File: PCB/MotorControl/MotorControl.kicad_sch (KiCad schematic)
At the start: 23 parts, among them J1 Conn_01x03_Pin, J2 Conn_01x03_Pin, J3 Conn_01x03_Pin, J4 Conn_01x03_Pin, J5 Conn_01x05_Pin, J6 USB_C_Receptacle_USB2.0_14P, J7 Conn_01x03_Pin, J8 Conn_01x02_Pin, U1 PCA9685PW, U2 NORA-W106-00B, U3 TC1262-33, U4 STM32L031K6Tx

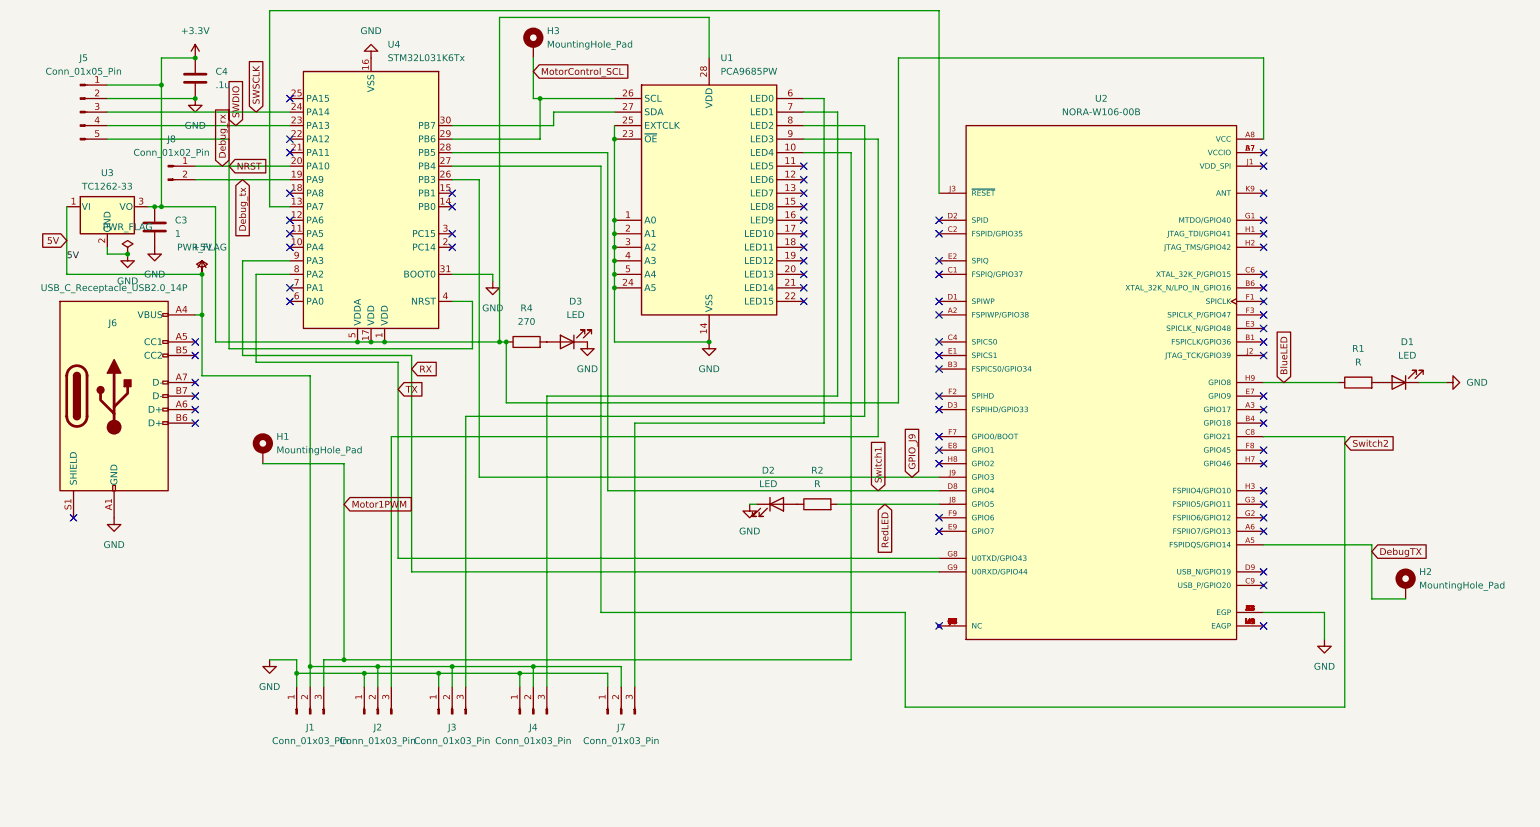
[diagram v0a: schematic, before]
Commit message: Motor
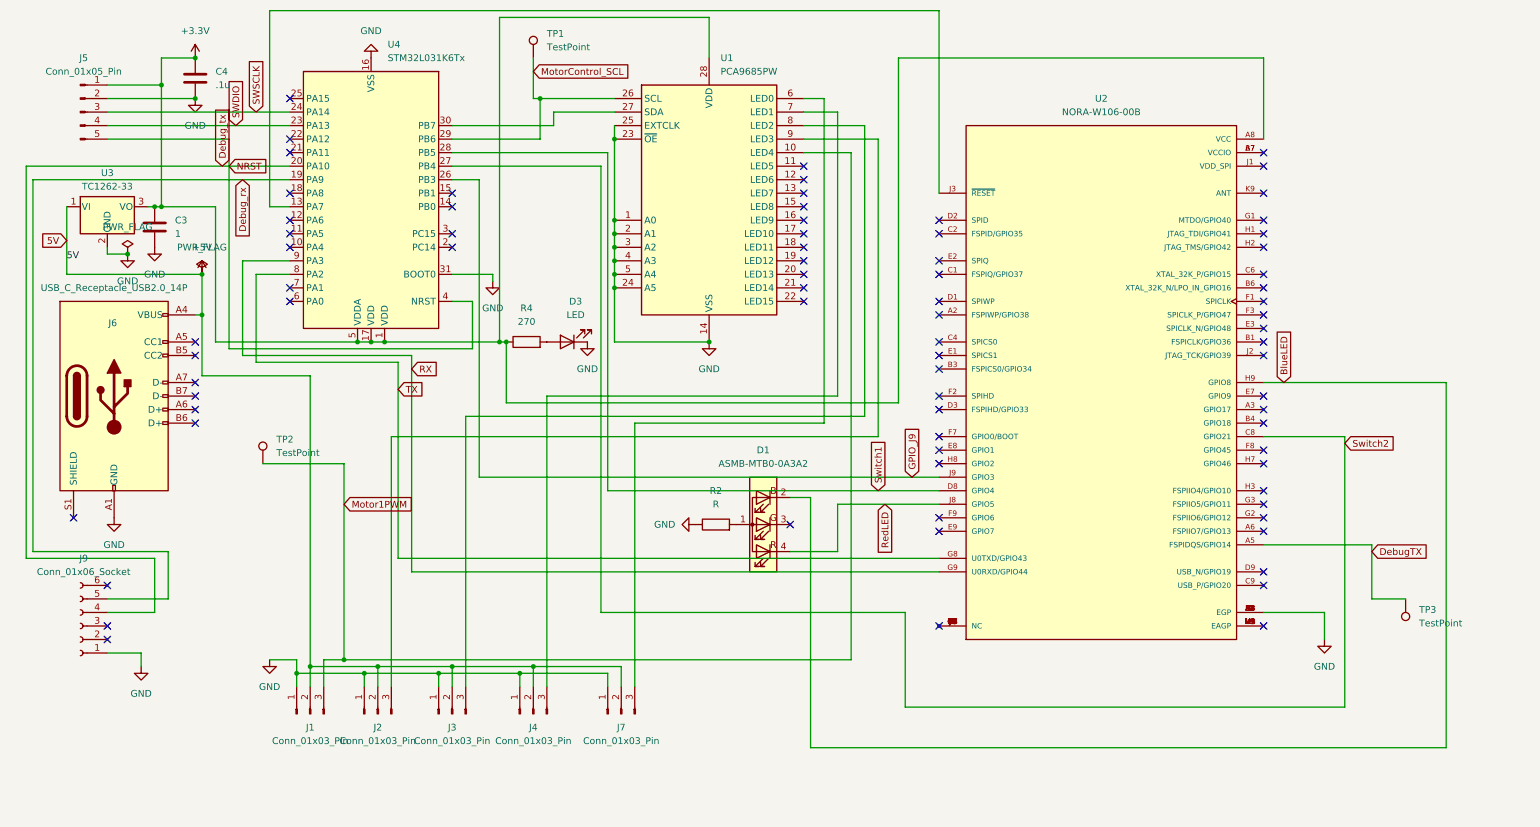
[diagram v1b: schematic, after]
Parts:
- removed D1, D2: LED, LED_SMD:LED_1206_3216Metric_Pad1.42x1.75mm_HandSolder, symbol Device:LED
- removed H1, H2, H3: MountingHole_Pad, MountingHole:MountingHole_4.5mm_Pad, symbol Mechanical:MountingHole_Pad
- removed J8: Conn_01x02_Pin, Connector_PinHeader_2.54mm:PinHeader_1x02_P2.54mm_Vertical, symbol Connector:Conn_01x02_Pin
- removed R1: R, Resistor_SMD:R_0805_2012Metric_Pad1.20x1.40mm_HandSolder, symbol Device:R
- added D1: ASMB-MTB0-0A3A2, LED_SMD:LED_Avago_PLCC4_3.2x2.8mm_CW, symbol LED:ASMB-MTB0-0A3A2
- added J9: Conn_01x06_Socket, Connector_PinSocket_2.54mm:PinSocket_1x06_P2.54mm_Vertical, symbol Connector:Conn_01x06_Socket
- added TP1, TP2, TP3: TestPoint, TestPoint:TestPoint_Pad_2.5x2.5mm, symbol Connector:TestPoint
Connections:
- net BlueLED: now also D1.2 (BK)
- net DebugTX: now also TP3.1
- net Debug_rx: now also U4.19 (PA9), J9.5 (Pin_5); no longer J5.5 (Pin_5), U4.20 (PA10), U4.4 (NRST)
- net Debug_tx: now also J5.5 (Pin_5), U4.20 (PA10), U4.4 (NRST), J9.4 (Pin_4); no longer U4.19 (PA9)
- net GND: now also R2.1, J9.1 (Pin_1)
- net Motor1PWM: now also TP2.1
- net MotorControl_SCL: now also TP1.1
- net RedLED: now also D1.4 (RK); no longer R2.2
- new net: D1.1 (A), R2.2
- no-connect marks 73 -> 77
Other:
- moved on the sheet: R2

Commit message: wasd
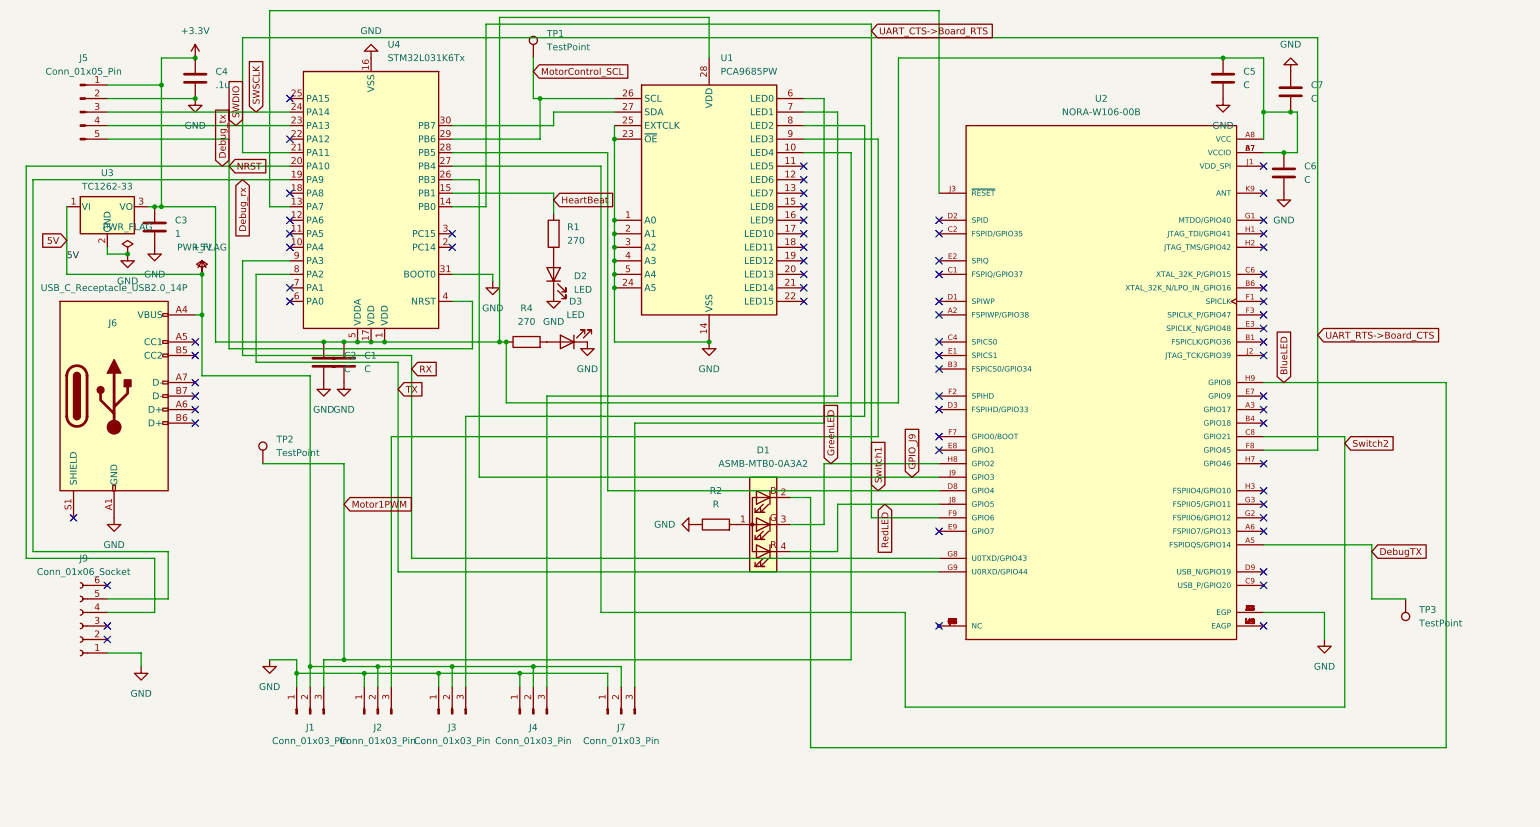
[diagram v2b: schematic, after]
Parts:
- added C1, C2, C5, C6, C7: C, Capacitor_SMD:C_0504_1310Metric_Pad0.83x1.28mm_HandSolder, symbol Device:C
- added D2: LED, LED_SMD:LED_1206_3216Metric_Pad1.42x1.75mm_HandSolder, symbol Device:LED
- added R1: 270, Resistor_SMD:R_0805_2012Metric_Pad1.20x1.40mm_HandSolder, symbol Device:R
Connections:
- net +3.3V: now also U2.A7 (VCCIO), U2.B7 (VCCIO), C1.1, C2.1, C5.1, C6.1, C7.2
- net GND: now also C1.2, C2.2, C5.2, C6.2, C7.1, D2.1 (K)
- net RX: now also U2.G8 (U0TXD/GPIO43); no longer U2.G9 (U0RXD/GPIO44)
- net TX: now also U2.G9 (U0RXD/GPIO44); no longer U2.G8 (U0TXD/GPIO43)
- net GreenLED: now reaches D1.3 (GK)
- net GreenLED: now also U2.H8 (GPIO2)
- net UART_RTS->Board_CTS: now reaches U2.F8 (GPIO45)
- net UART_RTS->Board_CTS: now also U4.21 (PA11)
- net UART_CTS->Board_RTS: now reaches U2.F9 (GPIO6)
- net UART_CTS->Board_RTS: now also U4.14 (PB0)
- net HeartBeat: now reaches U4.15 (PB1)
- net HeartBeat: now also R1.2
- new net: D2.2 (A), R1.1
- no-connect marks 77 -> 69

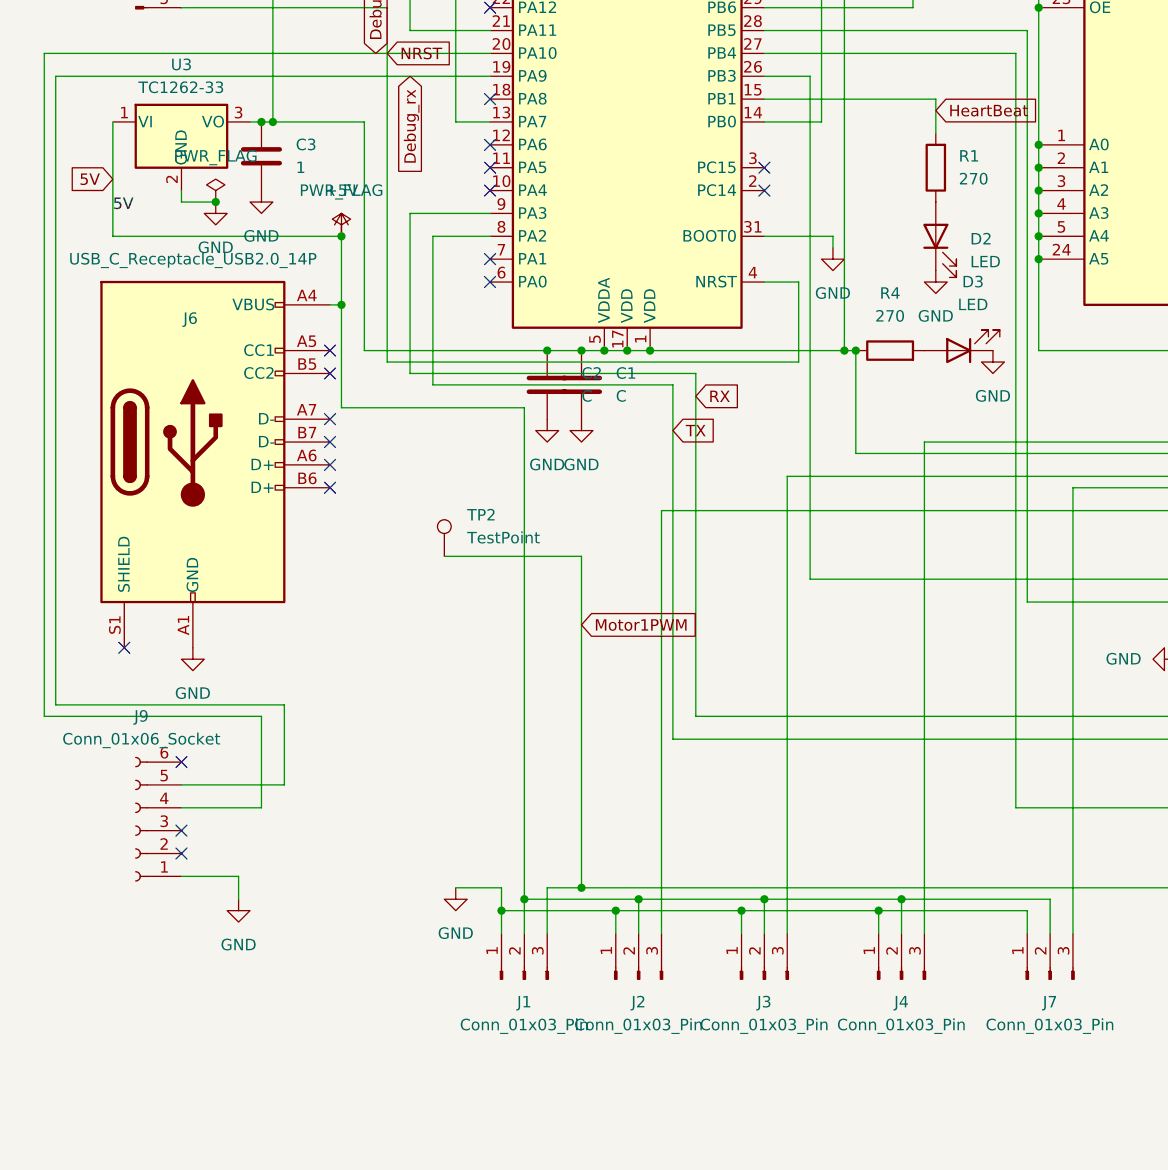
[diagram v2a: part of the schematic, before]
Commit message: wasd
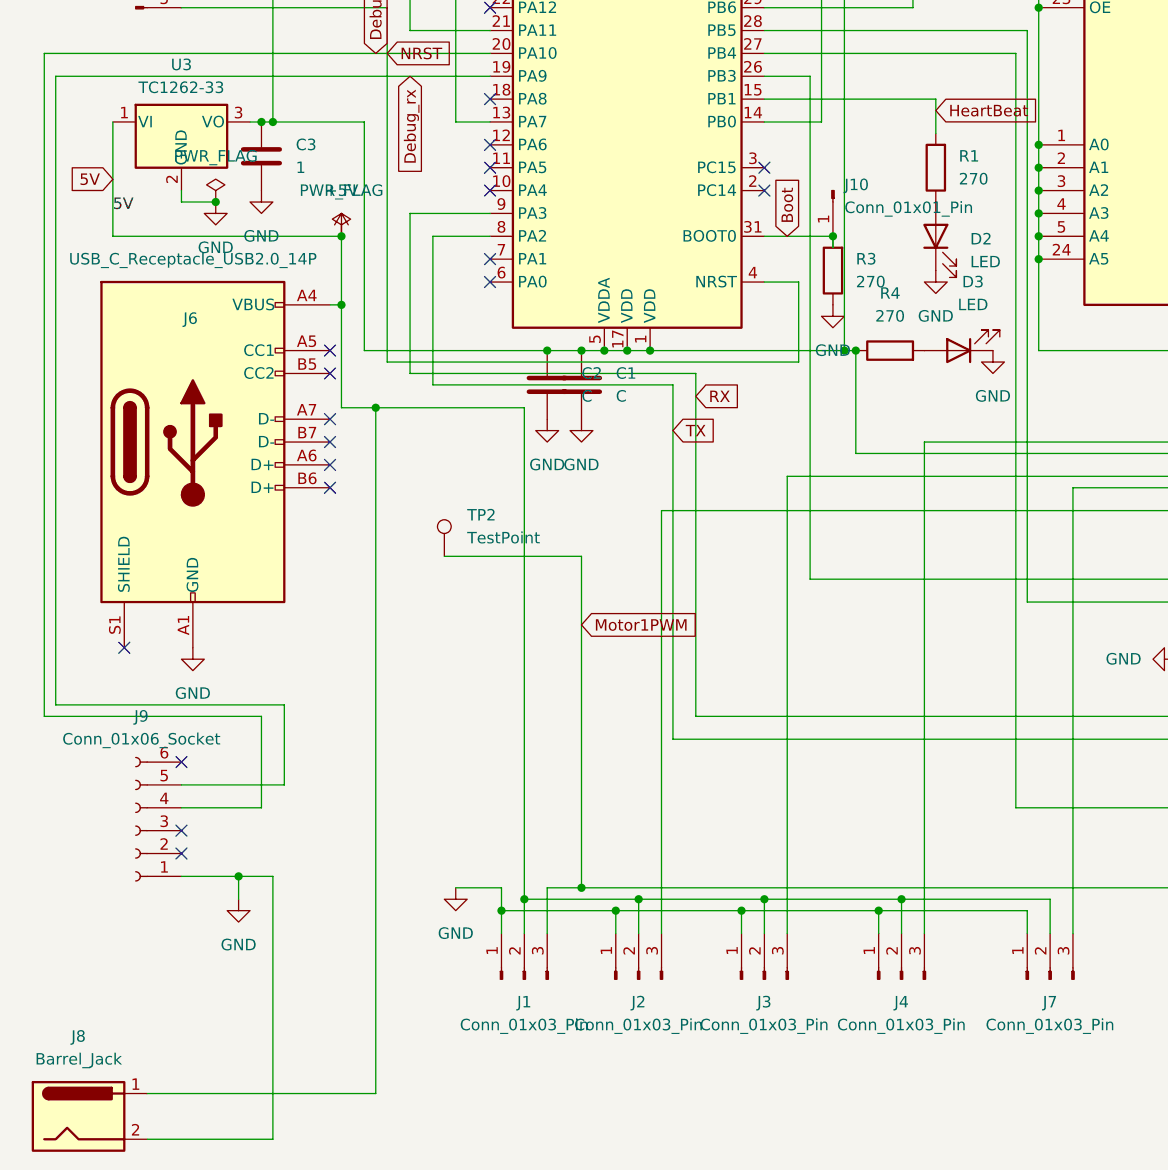
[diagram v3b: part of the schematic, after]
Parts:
- added J10: Conn_01x01_Pin, Connector_PinHeader_2.54mm:PinHeader_1x01_P2.54mm_Vertical, symbol Connector:Conn_01x01_Pin
- added J8: Barrel_Jack, Connector_BarrelJack:BarrelJack_CUI_PJ-063AH_Horizontal, symbol Connector:Barrel_Jack
- added R3: 270, Resistor_SMD:R_0805_2012Metric_Pad1.20x1.40mm_HandSolder, symbol Device:R
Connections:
- net +5V: now also J8.1
- net GND: now also J8.2, R3.1; no longer U4.31 (BOOT0)
- new net Boot: J10.1 (Pin_1), R3.2, U4.31 (BOOT0)
